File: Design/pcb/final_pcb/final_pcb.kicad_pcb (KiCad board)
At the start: 2 copper layers, 87 x 41 mm, 33 parts, among them J1 USB_C_Receptacle_USB2.0_14P, J2 Screw_Terminal_01x02, J3 Screw_Terminal_01x02, J5 Conn_01x05_Pin, Q1 NMOS, Q2 NMOS, U1 IR2184, U2 PIC32MZ2048EFM144-I/PH, U3 LM7812_TO220, U4 LM1117DT-3.3, Y1 SG-8002CA

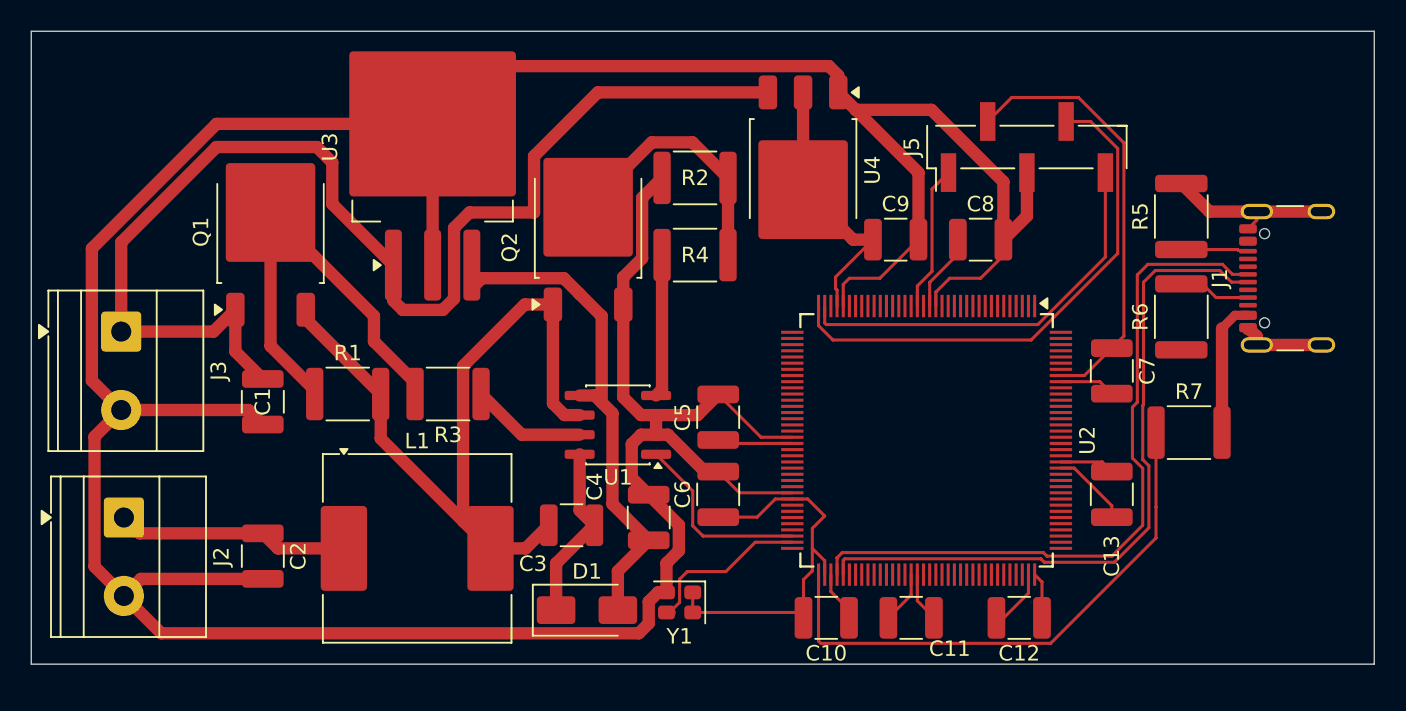
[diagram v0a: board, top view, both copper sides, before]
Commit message: Final PCB
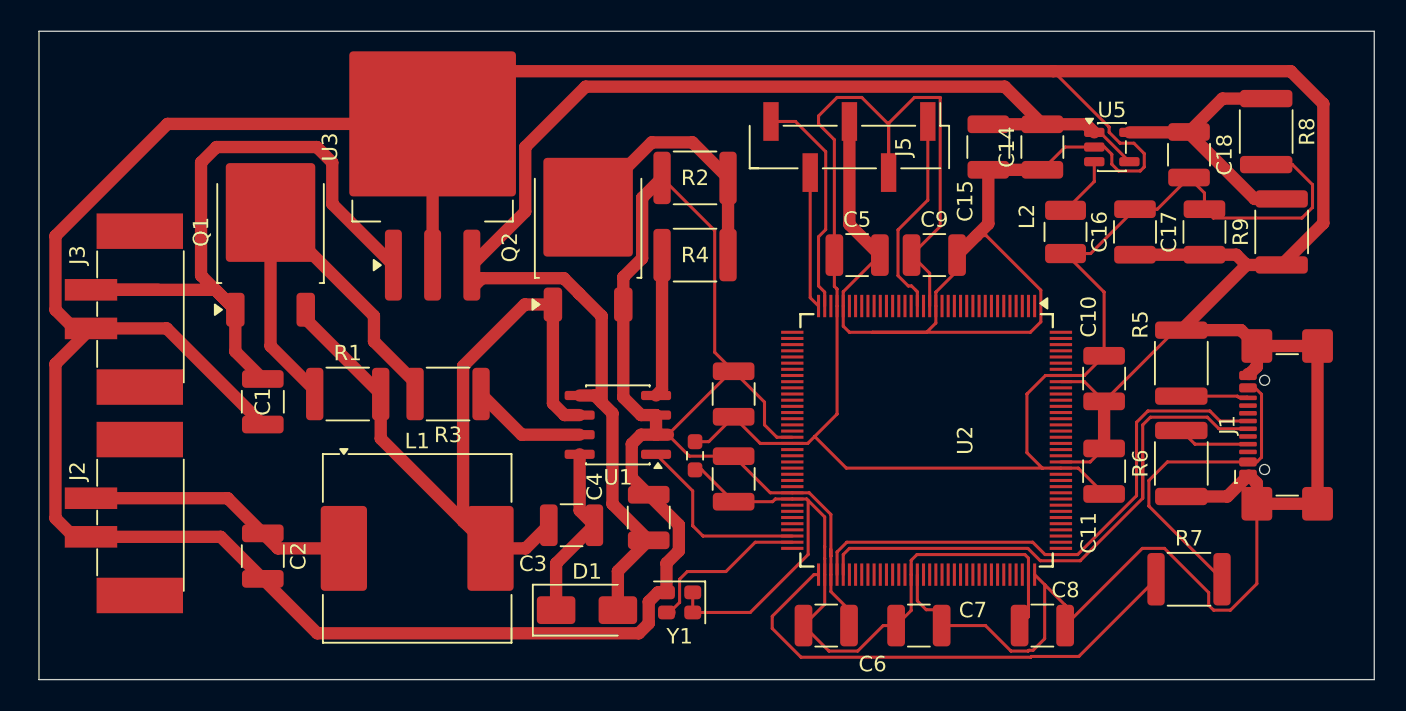
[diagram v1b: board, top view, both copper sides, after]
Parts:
- removed U4: LM1117DT-3.3, Package_TO_SOT_SMD:TO-252-3_TabPin2
- added C14: 10u, Capacitor_SMD:C_1210_3225Metric, F.Cu at (137.5, 70.5)
- added C15: 0.1u, Capacitor_SMD:C_1210_3225Metric, F.Cu at (134.0, 70.5)
- added C16: 10u, Capacitor_SMD:C_1210_3225Metric, F.Cu at (143.5, 76.0)
- added C17: 10u, Capacitor_SMD:C_1210_3225Metric, F.Cu at (148.0, 76.0)
- added C18: 0.1u, Capacitor_SMD:C_1210_3225Metric, F.Cu at (147.0, 71.0)
- added L2: L, Inductor_SMD:L_1210_3225Metric, F.Cu at (139.0, 76.0)
- added R10: 0, Resistor_SMD:R_0603_1608Metric_Pad0.98x0.95mm_HandSolder, F.Cu at (115.0, 90.5)
- added R8: 6.19k, Resistor_SMD:R_1812_4532Metric, F.Cu at (152.0, 69.5)
- added R9: 20k, Resistor_SMD:R_1812_4532Metric, F.Cu at (153.0, 76.0)
- added U5: TPS560200, Package_TO_SOT_SMD:SOT-23-5, F.Cu at (142.0, 70.5)
- J1: footprint Connector_USB:USB_C_Receptacle_GCT_USB4105-xx-A_16P_TopMnt_Horizontal -> Connector_USB:USB_C_Receptacle_GCT_USB4110
- J2, J3: footprint TerminalBlock_Phoenix:TerminalBlock_Phoenix_MKDS-1,5-2-5.08_1x02_P5.08mm_Horizontal -> TerminalBlock_Phoenix:TerminalBlock_Phoenix_PTSM-0,5-2-2,5-V-SMD_1x02-1MP_P2.50mm_Vertical
- U3: value LM7812_TO220 -> LM7812
- moved C13 25.3 mm to (117.5, 86.5)
- moved C8 25.3 mm to (137.5, 101.5)
- moved C10 23.8 mm to (141.5, 85.5), turned to 90 degrees
- moved C7 20.7 mm to (129.5, 101.5), turned to 0 degrees
- moved C12 20.6 mm to (117.5, 92.0), turned to -90 degrees
- moved C11 15.7 mm to (141.5, 91.5), turned to 90 degrees
- moved C5 13.8 mm to (125.5, 77.5), turned to 0 degrees
- moved J5 11.5 mm to (125.0, 70.5), turned to -90 degrees
- moved C6 11.0 mm to (123.5, 101.5), turned to 0 degrees
- moved J1 9.50 mm to (154.5, 88.5)
- moved R5 9.50 mm to (146.5, 84.5)
- moved R6 9.50 mm to (146.5, 91.0)
- moved R7 9.50 mm to (147.0, 98.5)
- moved C9 2.69 mm to (130.5, 77.5)
- moved J3 1.47 mm to (78.0, 81.0)
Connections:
- net +12V renamed 12v
- net 5v renamed LM_input
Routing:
- net GND: track 279.3 -> 453.0 mm
- net 3.3V: track 93.9 -> 182.0 mm
- net 12v: track 32.5 -> 87.8 mm
- net LM_input: track 81.4 -> 47.6 mm
- net 4: track 34.2 -> 8.87 mm
- net Net-(U5-FB): track 0.00 -> 17.6 mm
- net Net-(J1-VBUS-PadA4): track 8.79 -> 21.4 mm
- net 5: track 26.6 -> 14.7 mm
- net D-: track 46.3 -> 35.6 mm
- net D+: track 45.3 -> 37.7 mm
- net Net-(U5-PH): track 0.00 -> 3.92 mm
- net 1: track 9.48 -> 13.4 mm
- net vbus: track 35.9 -> 32.6 mm
- net Net-(J2-Pin_1): track 15.1 -> 17.7 mm
- net Net-(J1-CC1): track 3.33 -> 4.69 mm
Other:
- board size 87 x 41 mm -> 86.5 x 42 mm
